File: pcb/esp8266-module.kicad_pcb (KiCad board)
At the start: 2 copper layers, 37.4 x 38.3 mm, 15 parts, among them U1 ESP-12E

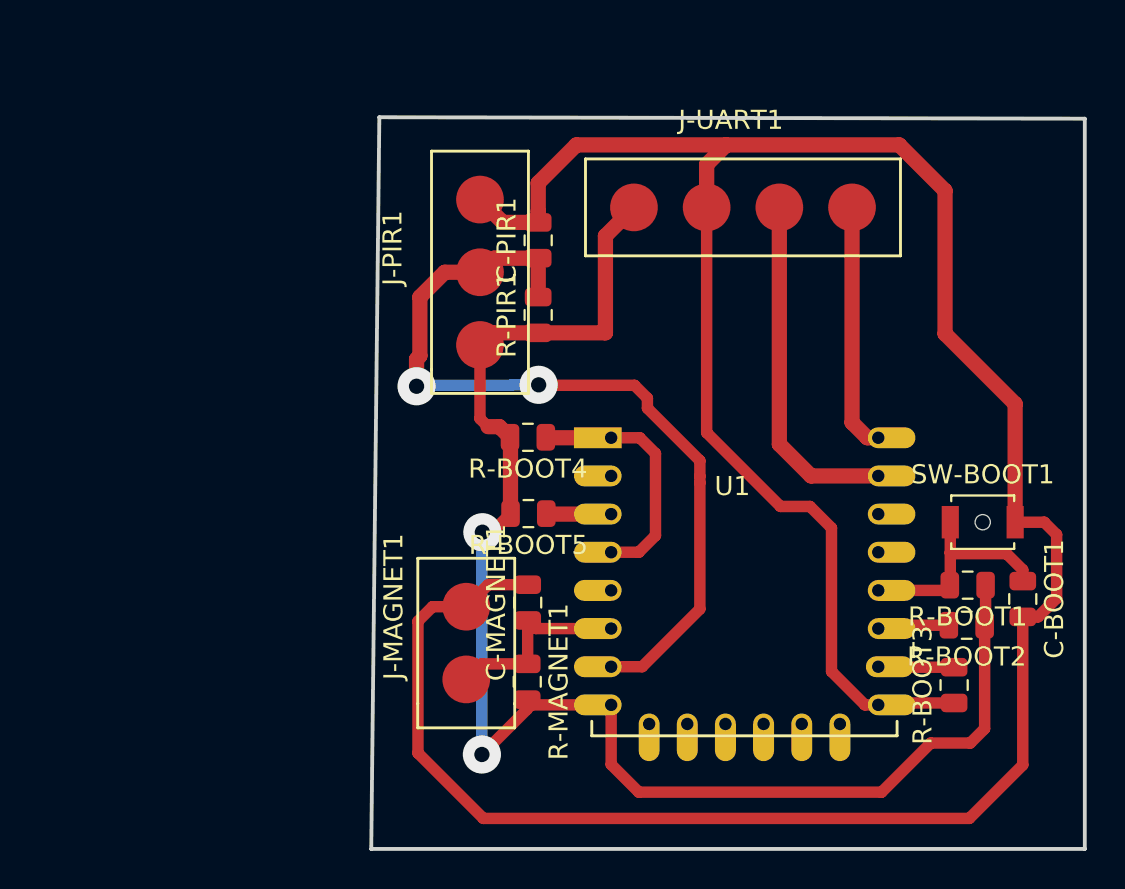
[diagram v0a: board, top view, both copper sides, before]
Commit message: re-map I/O
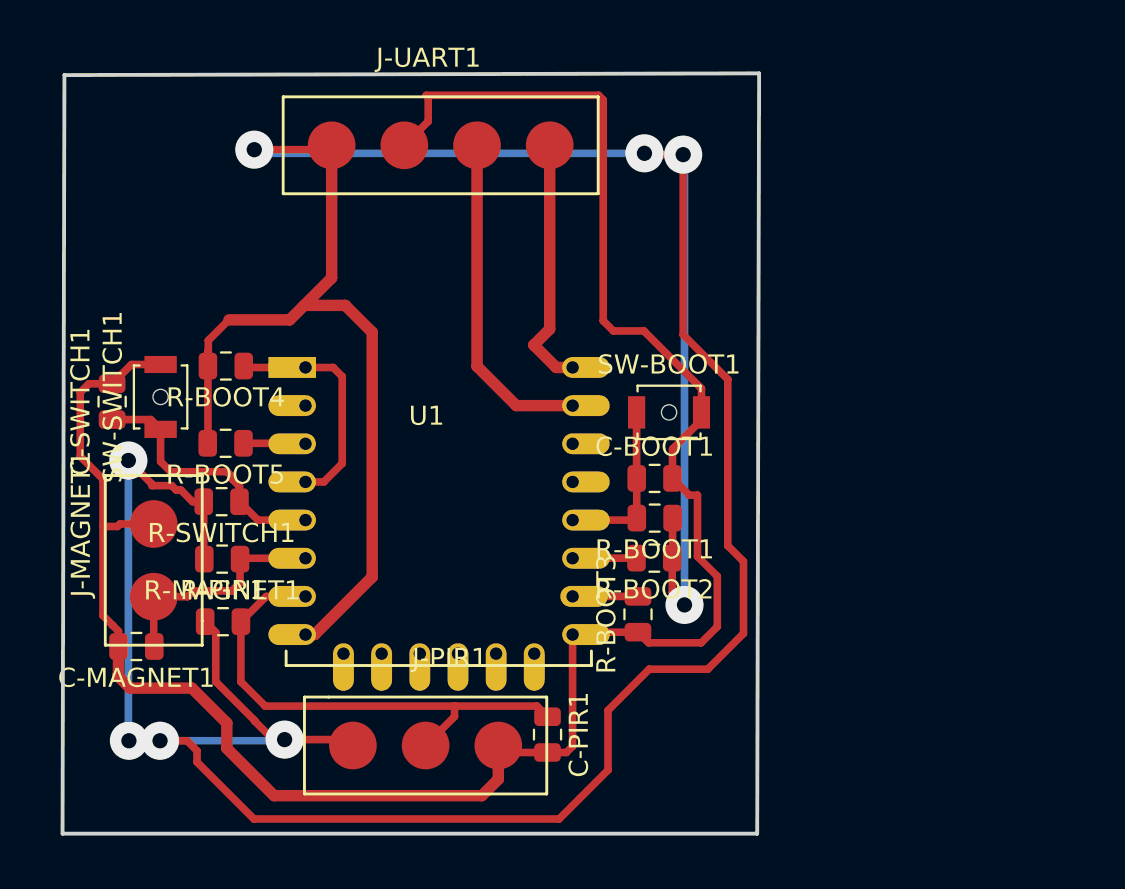
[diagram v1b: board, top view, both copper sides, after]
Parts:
- added C-SWITCH1: C, Capacitor_SMD:C_0805_2012Metric, F.Cu at (38.8, 53.4)
- added R-SWITCH1: 10K, Resistor_SMD:R_0805_2012Metric, F.Cu at (44.6, 58.6)
- added SW-SWITCH1: SW_Push, Button_Switch_SMD:SW_SPST_B3U-1000P-B, F.Cu at (41.4, 53.1)
- moved C-PIR1 25.9 mm to (61.6, 70.8), turned to 270 degrees
- moved R-PIR1 23.1 mm to (44.6, 64.9), turned to 0 degrees
- moved J-PIR1 21.3 mm to (56.5, 66.3), turned to 0 degrees
- moved C-MAGNET1 20.6 mm to (40.1, 66.2), turned to 180 degrees
- moved C-BOOT1 20.3 mm to (67.3, 57.4), turned to 0 degrees
- moved SW-BOOT1 17.4 mm to (68.0, 53.9)
- moved R-MAGNET1 17.2 mm to (44.6, 61.6), turned to 180 degrees
- moved R-BOOT3 17.0 mm to (66.4, 64.5)
- moved J-MAGNET1 16.9 mm to (35.9, 61.0)
- moved R-BOOT1 16.8 mm to (67.3, 59.5)
- moved R-BOOT2 16.7 mm to (67.2, 61.6)
- moved U1 16.4 mm to (49.0, 51.6)
- moved R-BOOT5 16.3 mm to (44.8, 55.5)
- moved R-BOOT4 16.3 mm to (44.8, 51.5)
- moved J-UART1 16.2 mm to (55.4, 34.8)
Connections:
- U1 pad 5: Net-(U1-Pad5) -> /GPIO_14
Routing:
- net VDD: track 78.0 -> 204.7 mm, vias 2 -> 8
- net GND: track 149.9 -> 112.0 mm
- net /GPIO_13: track 44.3 -> 26.6 mm, vias 2 -> 0
- net /GPIO_14: track 0.00 -> 13.8 mm
- net /GPIO_0: track 11.9 -> 8.95 mm
- net /GPIO_12: track 10.5 -> 12.1 mm
- net /RX: track 18.3 -> 17.4 mm
- net /nRST: track 13.1 -> 12.3 mm
- net Net-(R-BOOT3-Pad2): track 3.99 -> 3.42 mm
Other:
- board size 37.4 x 38.3 mm -> 36.5 x 39.9 mm
